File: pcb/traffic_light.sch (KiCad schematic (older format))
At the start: 51 parts, among them Q1 BS170, Q2 BS170, Q3 BS170, SW1 Power_Switch, U1 ESP-12F, U2 AMS1117-3.3

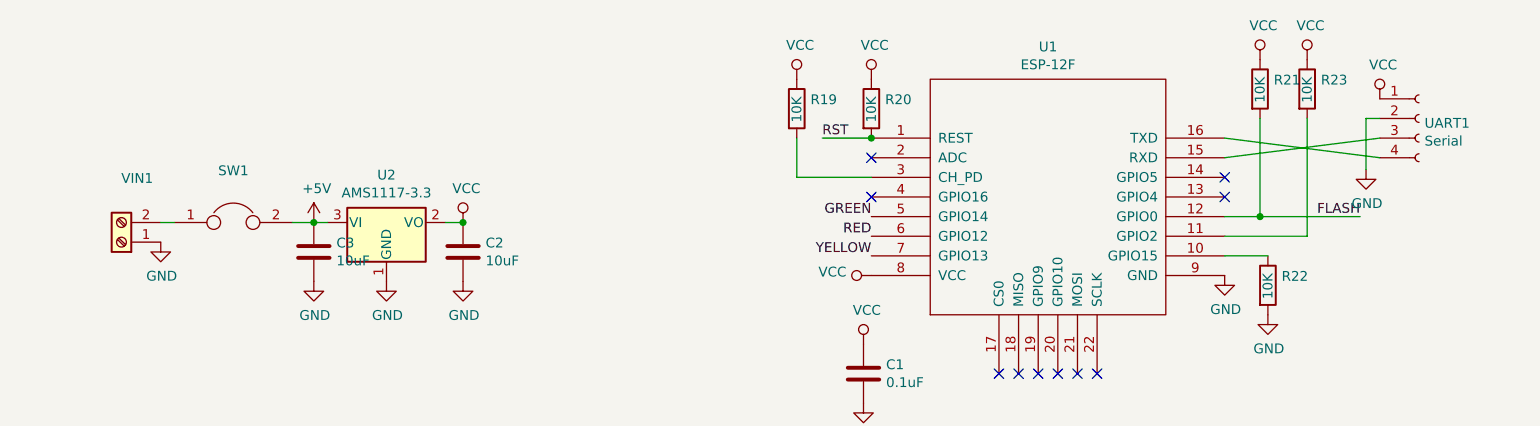
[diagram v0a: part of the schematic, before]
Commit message: Minor PCB improvements
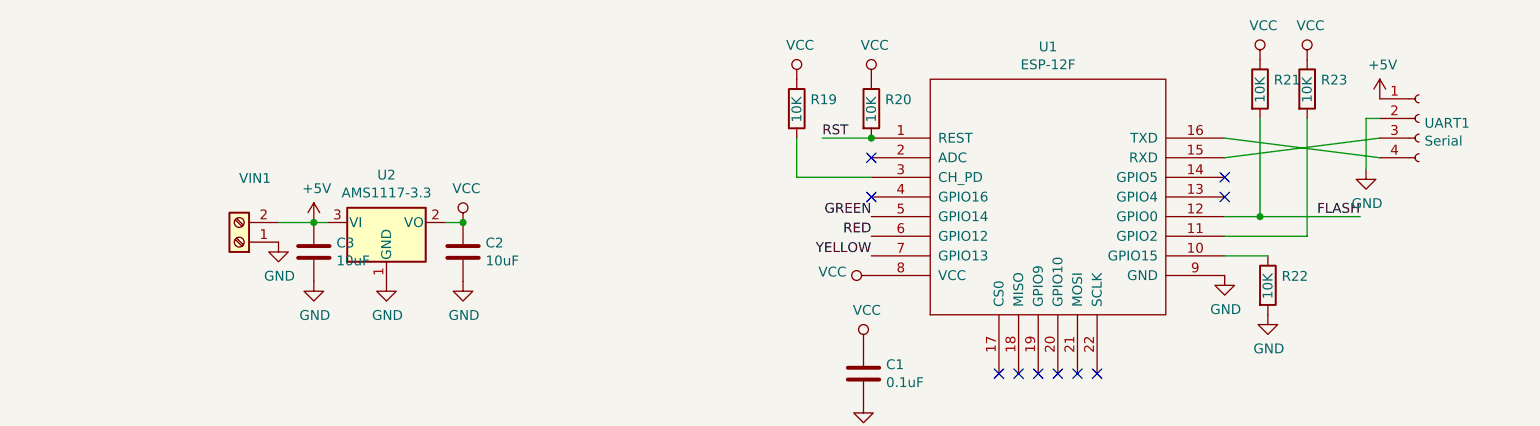
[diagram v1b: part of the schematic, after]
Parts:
- removed SW1: Power_Switch, Connector_PinHeader_2.54mm:PinHeader_1x02_P2.54mm_Vertical, symbol Device:Jumper
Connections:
- net +5V: now also UART1.1 (Pin_1), VIN1.2 (Pin_2)
- net VCC: no longer UART1.1 (Pin_1)
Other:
- moved on the sheet: VIN1
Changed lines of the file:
@@
 EESchema Schematic File Version 4
 LIBS:traffic_light-cache
-EELAYER 26 0
+EELAYER 29 0
 EELAYER END
 $Descr A4 11693 8268
@@
 $EndComp
 $Comp
-L power:VCC #PWR0121
-U 1 1 5C0BD195
-P 8020 1820
-F 0 "#PWR0121" H 8020 1670 50  0001 C CNN
-F 1 "VCC" H 8037 1993 50  0000 C CNN
-F 2 "" H 8020 1820 50  0001 C CNN
-F 3 "" H 8020 1820 50  0001 C CNN
-	1    8020 1820
-	1    0    0    -1
-$EndComp
-$Comp
 L power:GND #PWR0122
 U 1 1 5C0BD64D
@@
 L Connector:Screw_Terminal_01x02 VIN1
 U 1 1 5C0DA213
-P 1610 2550
-F 0 "VIN1" H 1530 2225 50  0000 C CNN
-F 1 "Power" H 1530 2316 50  0001 C CNN
-F 2 "Connector_PinHeader_2.54mm:PinHeader_1x02_P2.54mm_Vertical" H 1610 2550 50  0001 C CNN
-F 3 "~" H 1610 2550 50  0001 C CNN
-	1    1610 2550
+P 2210 2550
+F 0 "VIN1" H 2130 2225 50  0000 C CNN
+F 1 "Power" H 2130 2316 50  0001 C CNN
+F 2 "Connector_PinHeader_2.54mm:PinHeader_1x02_P2.54mm_Vertical" H 2210 2550 50  0001 C CNN
+F 3 "~" H 2210 2550 50  0001 C CNN
+	1    2210 2550
 	-1   0    0    1
 $EndComp
@@
 L power:GND #PWR0126
 U 1 1 5C0DD276
-P 1810 2550
-F 0 "#PWR0126" H 1810 2300 50  0001 C CNN
-F 1 "GND" H 1815 2377 50  0000 C CNN
-F 2 "" H 1810 2550 50  0001 C CNN
-F 3 "" H 1810 2550 50  0001 C CNN
-	1    1810 2550
+P 2410 2550
+F 0 "#PWR0126" H 2410 2300 50  0001 C CNN
+F 1 "GND" H 2415 2377 50  0000 C CNN
+F 2 "" H 2410 2550 50  0001 C CNN
+F 3 "" H 2410 2550 50  0001 C CNN
+	1    2410 2550
 	1    0    0    -1
 $EndComp
@@
 	1    0    0    -1
 $EndComp
-$Comp
-L Device:Jumper SW1
-U 1 1 5C0EB53D
-P 2180 2450
-F 0 "SW1" H 2180 2714 50  0000 C CNN
-F 1 "Power_Switch" H 2180 2623 50  0001 C CNN
-F 2 "Connector_PinHeader_2.54mm:PinHeader_1x02_P2.54mm_Vertical" H 2180 2450 50  0001 C CNN
-F 3 "~" H 2180 2450 50  0001 C CNN
-	1    2180 2450
-	1    0    0    -1
-$EndComp
 Wire Wire Line
 	2660 2450 2590 2450
-Wire Wire Line
-	2480 2450 2590 2450
 Connection ~ 2590 2450
-Wire Wire Line
-	1810 2450 1880 2450
 $Comp
 L power:+5V #PWR0103
@@
 	1    0    0    -1
 $EndComp
+$Comp
+L power:+5V #PWR0121
+U 1 1 5CC9FB36
+P 8020 1820
+F 0 "#PWR0121" H 8020 1670 50  0001 C CNN
+F 1 "+5V" H 8035 1993 50  0000 C CNN
+F 2 "" H 8020 1820 50  0001 C CNN
+F 3 "" H 8020 1820 50  0001 C CNN
+	1    8020 1820
+	1    0    0    -1
+$EndComp
+Wire Wire Line
+	2410 2450 2590 2450
 $EndSCHEMATC
